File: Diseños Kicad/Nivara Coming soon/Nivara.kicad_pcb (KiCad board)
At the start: 2 copper layers, 107 x 87.7 mm, 20 parts, among them J1 Screw_Terminal_01x02, J12 Screw_Terminal_01x04, J13 Screw_Terminal_01x02, J14 Screw_Terminal_01x06, J2 Screw_Terminal_01x04, J3 Screw_Terminal_01x02, J4 Screw_Terminal_01x02, J5 Screw_Terminal_01x03, J6 Screw_Terminal_01x02, J9 Screw_Terminal_01x03, U1 ESP32-S3-WROOM-1, U2 AP63203WU

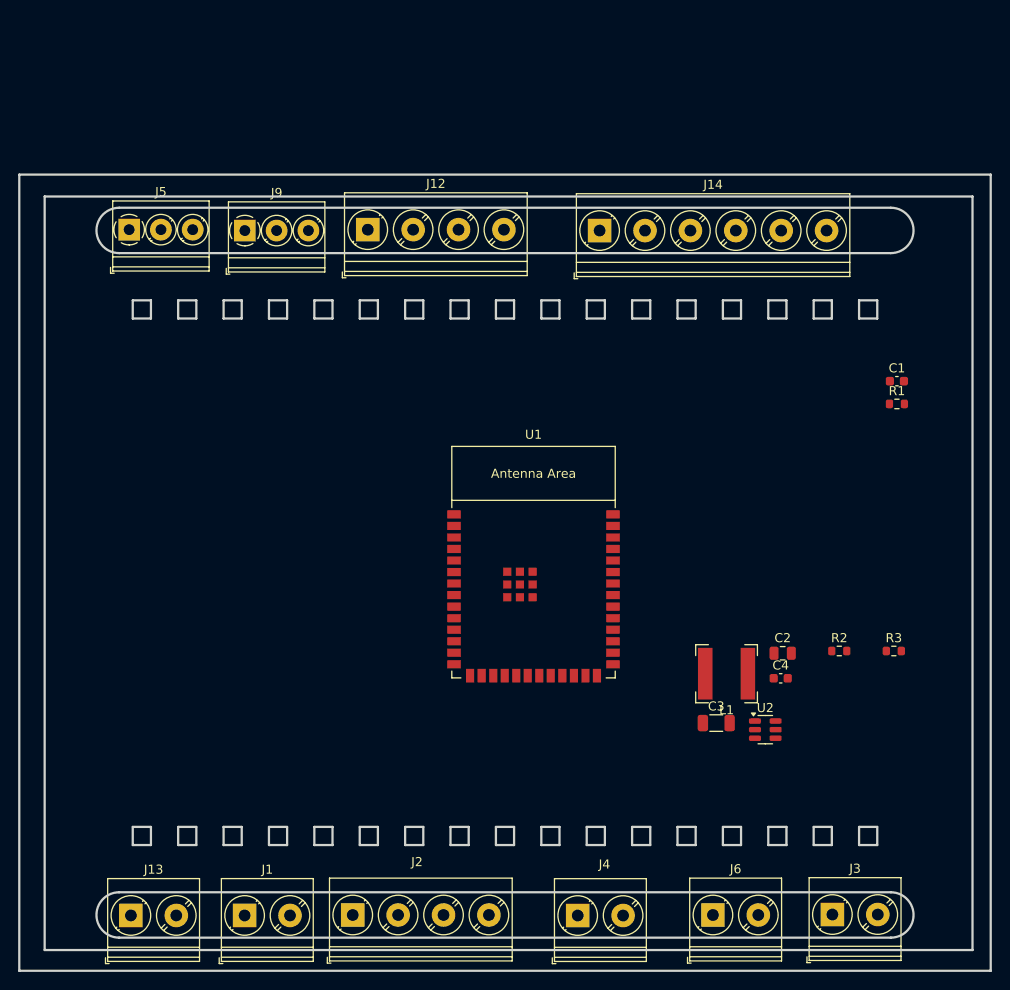
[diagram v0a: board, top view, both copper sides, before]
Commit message: UPDATE TAREA
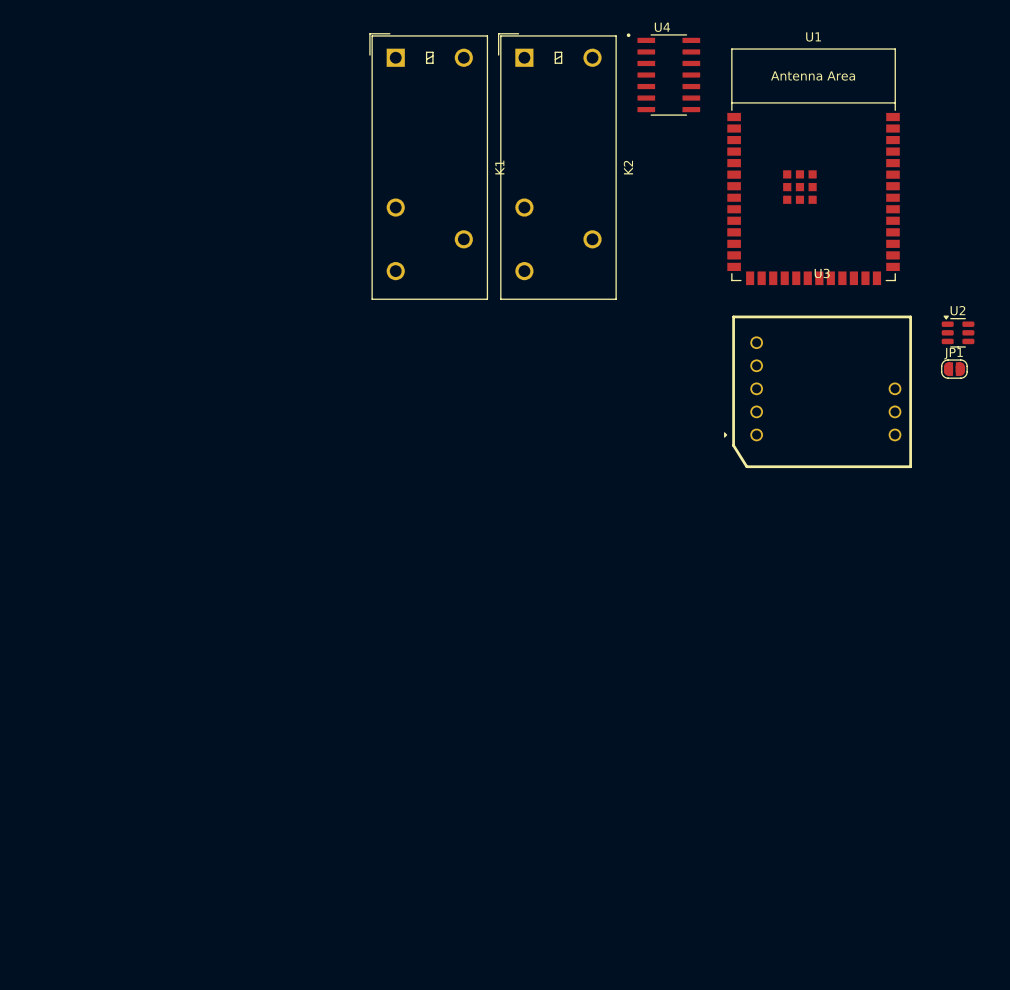
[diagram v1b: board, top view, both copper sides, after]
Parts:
- removed C1: 1uf, Capacitor_SMD:C_0603_1608Metric
- removed C2: 22uf, Capacitor_SMD:C_0805_2012Metric
- removed C3: 10mf, Capacitor_SMD:C_1206_3216Metric
- removed C4: 100nf, Capacitor_SMD:C_0603_1608Metric
- removed J1, J13, J3, J4, J6: Screw_Terminal_01x02, TerminalBlock_Phoenix:TerminalBlock_Phoenix_PT-1,5-2-5.0-H_1x02_P5.00mm_Horizontal
- removed J12, J2: Screw_Terminal_01x04, TerminalBlock_Phoenix:TerminalBlock_Phoenix_PT-1,5-4-5.0-H_1x04_P5.00mm_Horizontal
- removed J14: Screw_Terminal_01x06, TerminalBlock_Phoenix:TerminalBlock_Phoenix_PT-1,5-6-5.0-H_1x06_P5.00mm_Horizontal
- removed J5, J9: Screw_Terminal_01x03, TerminalBlock_Phoenix:TerminalBlock_Phoenix_PT-1,5-3-3.5-H_1x03_P3.50mm_Horizontal
- removed L1: L_Iron, Inductor_SMD:L_Bourns-SRN6028
- removed R1, R2, R3: R_US, Resistor_SMD:R_0603_1608Metric
- added JP1: SolderJumper_2_Open, Jumper:SolderJumper-2_P1.3mm_Open_RoundedPad1.0x1.5mm, F.Cu at (143.8, 91.0)
- added K1: G2RL-1, Relay_THT:Relay_SPDT_Omron_G2RL-1, F.Cu at (82.3, 56.7)
- added K2: G2RL-1, Relay_THT:Relay_SPDT_Omron_G2RL-1, F.Cu at (96.5, 56.7)
- added U3: ~, Riqi_Parts:YLPTEC RSM3485ECHT, F.Cu at (119.5, 101.8)
- added U4: ~, Riqi_Parts:SOIC127P600X172-14N, F.Cu at (112.4, 58.6)
- moved U1 53.5 mm to (128.3, 71.5)
- moved U2 48.6 mm to (144.2, 87.0)
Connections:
- U1 pad 36: /Board_ZorionX/Driver_RS485/UART_OUT -> /NIVARA_BOARD/RS485_INTERFACE/UART_RX
- U1 pad 37: /Board_ZorionX/Driver_RS485/UART_R_IN -> /NIVARA_BOARD/RS485_INTERFACE/UART_TX
- U2 pad 1: unconnected-(U2-FB-Pad1) -> Net-(JP1-A)
- U2 pad 2: unconnected-(U2-EN-Pad2) -> VCC
- U2 pad 3: unconnected-(U2-IN-Pad3) -> VCC
- U2 pad 4: unconnected-(U2-GND-Pad4) -> GND
- U2 pad 5: unconnected-(U2-SW-Pad5) -> Net-(U2-SW)
- U2 pad 6: unconnected-(U2-BST-Pad6) -> Net-(U2-BST)
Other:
- board outline removed
